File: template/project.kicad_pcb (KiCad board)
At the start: 2 copper layers, 7 parts

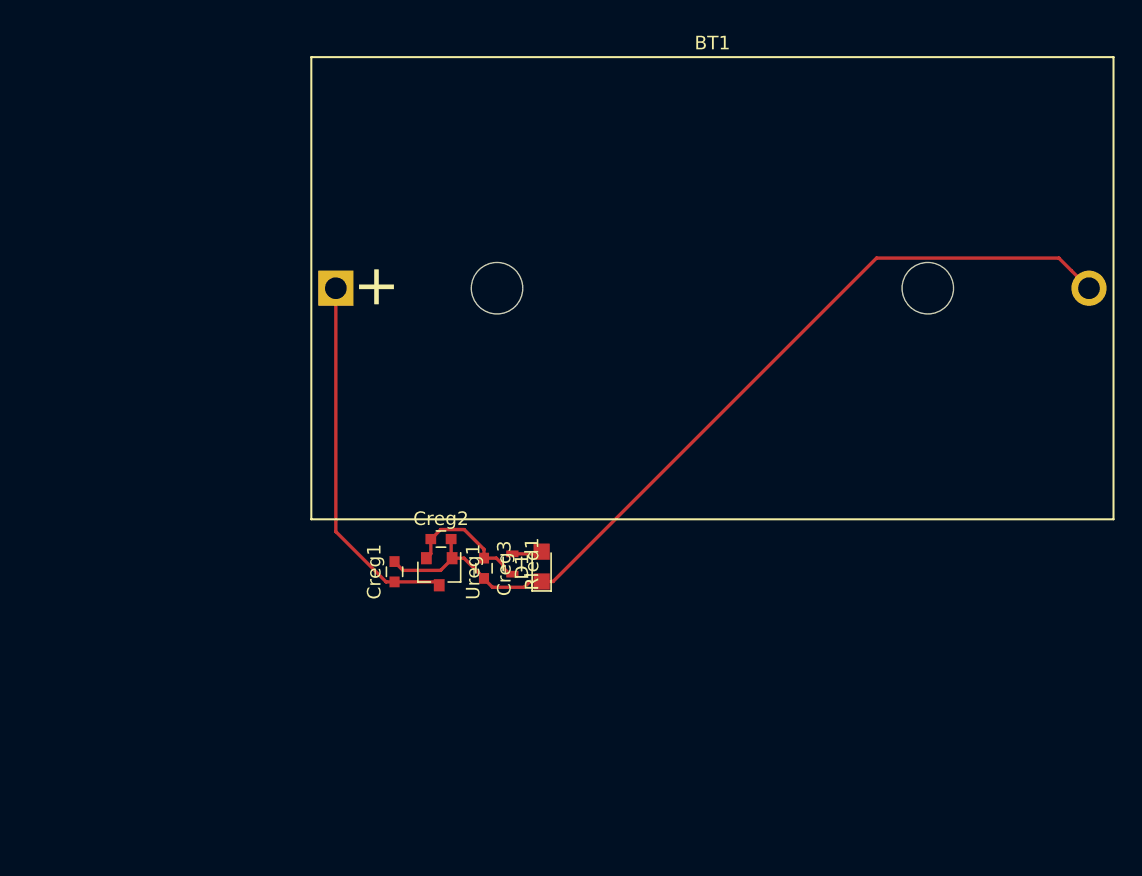
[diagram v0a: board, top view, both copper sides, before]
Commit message: Continued play with libraries
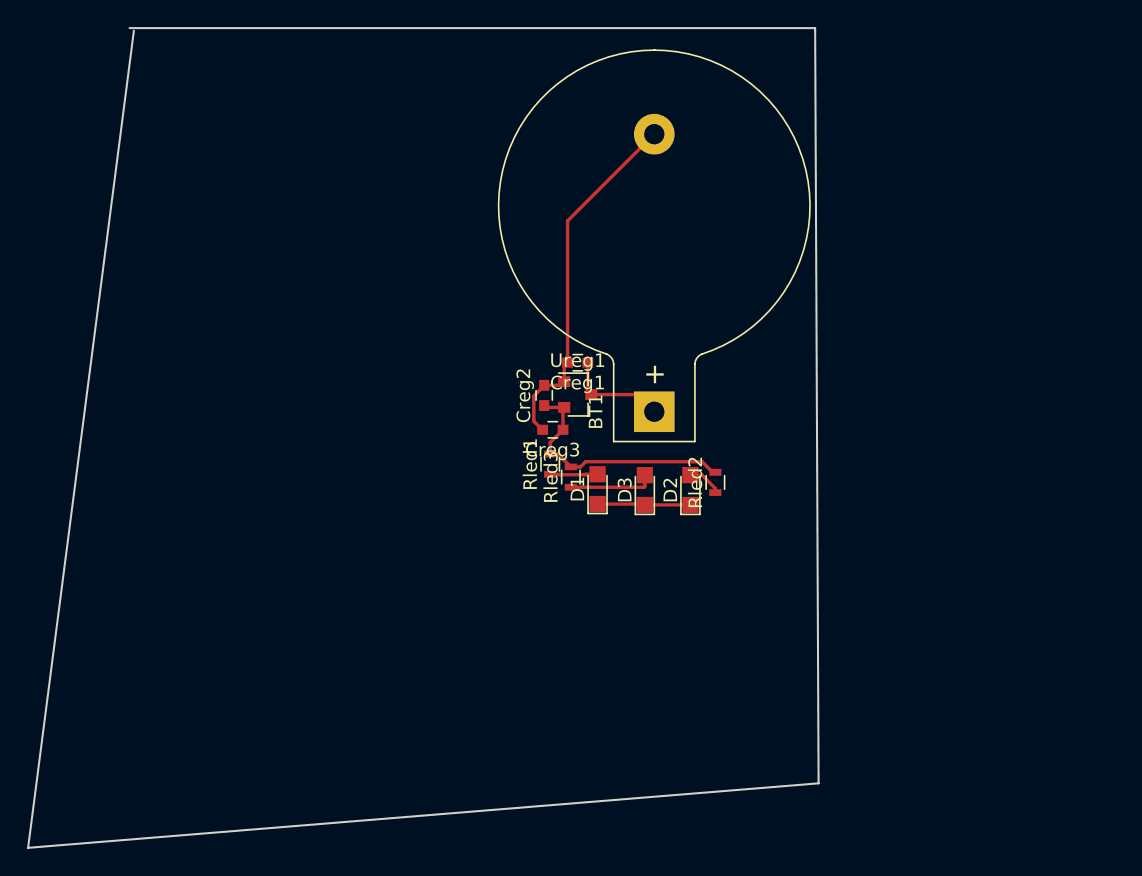
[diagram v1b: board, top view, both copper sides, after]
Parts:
- added D2: LED-B, LEDs:LED_0805, F.Cu at (183.6, 138.9)
- added D3: LED-R, LEDs:LED_0805, F.Cu at (180.3, 138.9)
- added Rled2: 499, Resistors_SMD:R_0603, F.Cu at (185.5, 138.3)
- added Rled3: 499, Resistors_SMD:R_0603, F.Cu at (174.8, 137.9)
- BT1: footprint Battery_Holders:Bulgin_BX0036_1xC -> Battery_Holders:Keystone_103_1x20mm-CoinCell
- D1: value LED-R -> LED-G
- moved BT1 25.2 mm to (181.0, 133.1), turned to 90 degrees
- moved Creg1 20.5 mm to (175.3, 129.5), turned to 180 degrees
- moved Ureg1 16.6 mm to (175.3, 131.8), turned to 0 degrees
- moved Creg2 13.1 mm to (172.8, 131.9), turned to 90 degrees
- moved Creg3 11.4 mm to (173.5, 134.4), turned to 180 degrees
- moved Rled1 7.88 mm to (173.3, 137.0), turned to 90 degrees
- moved D1 7.05 mm to (176.8, 138.8)
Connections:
- net /Sheet59D70135/V_IN renamed /reg/V_IN
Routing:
- net GND: track 65.3 -> 33.4 mm
- net /reg/V_IN: track 27.2 -> 7.63 mm
- net +3V3: track 9.72 -> 18.5 mm
- net Net-(D3-Pad2): track 0.00 -> 6.33 mm
- net Net-(D2-Pad2): track 0.00 -> 2.79 mm
- net Net-(D1-Pad2): track 2.23 -> 3.52 mm
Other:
- board outline added: 58.4 x 60.5 mm
